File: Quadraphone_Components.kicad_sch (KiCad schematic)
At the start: 40 parts, among them J1 Conn_01x10_Male, J2 Conn_01x10_Male, J3 Conn_01x10_Male, J4 Conn_01x10_Male, J5 Eurorack_10_pin_power, Q1 MMBT3904, U1 AMS1117-5.0, U14 LM4040DBZ-2.5, U3 MCP6002, U4 LM4040DBZ-5, U5 MCP6004, U8 74LV4066PW

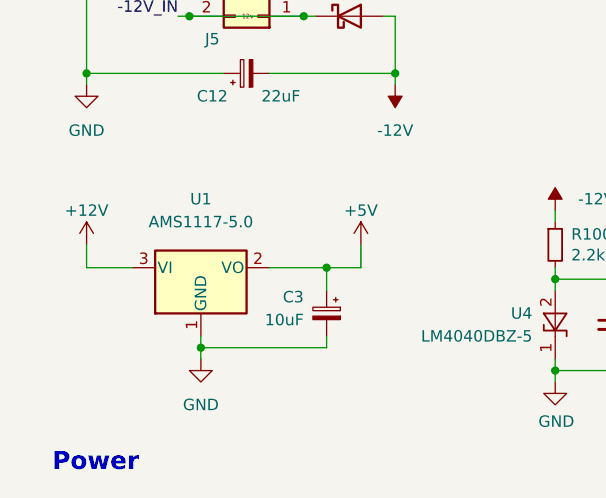
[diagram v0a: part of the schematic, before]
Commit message: Gerbers Prepared and Ordered
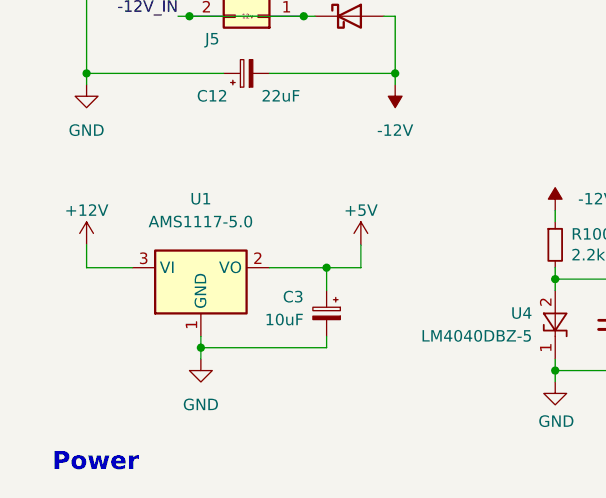
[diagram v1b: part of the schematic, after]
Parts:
- J1, J2, J3, J4: symbol Connector:Conn_01x10_Male -> Connector:Conn_01x10_Pin; now in the parts list
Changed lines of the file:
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@@
     )
   )
-  (symbol (lib_id "Connector:Conn_01x10_Male") (at 196.85 69.85 0) (unit 1)
-    (in_bom no) (on_board yes) (dnp no)
+  (symbol (lib_id "Connector:Conn_01x10_Pin") (at 196.85 69.85 0) (unit 1)
+    (in_bom yes) (on_board yes) (dnp no)
     (property "Reference" "J3" (at 197.485 54.61 0)
       (effects (font (size 1.27 1.27)))
@@
     )
   )
-  (symbol (lib_id "Connector:Conn_01x10_Male") (at 243.84 36.83 0) (unit 1)
-    (in_bom no) (on_board yes) (dnp no)
+  (symbol (lib_id "Connector:Conn_01x10_Pin") (at 243.84 36.83 0) (unit 1)
+    (in_bom yes) (on_board yes) (dnp no)
     (property "Reference" "J2" (at 244.475 21.59 0)
       (effects (font (size 1.27 1.27)))
@@
       (effects (font (size 1.27 1.27) italic) (justify left) hide)
     )
-    (property "Datasheet" "https://www.onsemi.com/pub/Collateral/2N3903-D.PDF" (at 256.54 135.89 0)
+    (property "Datasheet" "https://www.onsemi.com/pdf/datasheet/pzt3904-d.pdf" (at 256.54 135.89 0)
       (effects (font (size 1.27 1.27)) (justify left) hide)
     )
@@
     )
   )
-  (symbol (lib_id "Connector:Conn_01x10_Male") (at 243.84 69.85 0) (unit 1)
-    (in_bom no) (on_board yes) (dnp no)
+  (symbol (lib_id "Connector:Conn_01x10_Pin") (at 243.84 69.85 0) (unit 1)
+    (in_bom yes) (on_board yes) (dnp no)
     (property "Reference" "J4" (at 244.475 54.61 0)
       (effects (font (size 1.27 1.27)))
@@
     )
   )
-  (symbol (lib_id "Connector:Conn_01x10_Male") (at 196.85 36.83 0) (unit 1)
-    (in_bom no) (on_board yes) (dnp no)
+  (symbol (lib_id "Connector:Conn_01x10_Pin") (at 196.85 36.83 0) (unit 1)
+    (in_bom yes) (on_board yes) (dnp no)
     (property "Reference" "J1" (at 197.485 21.59 0)
       (effects (font (size 1.27 1.27)))
